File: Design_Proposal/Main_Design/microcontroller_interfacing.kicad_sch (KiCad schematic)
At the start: 9 parts, among them J12 Conn_01x02_Male, U3 CH340C, U4 M24C16-RMN6TP

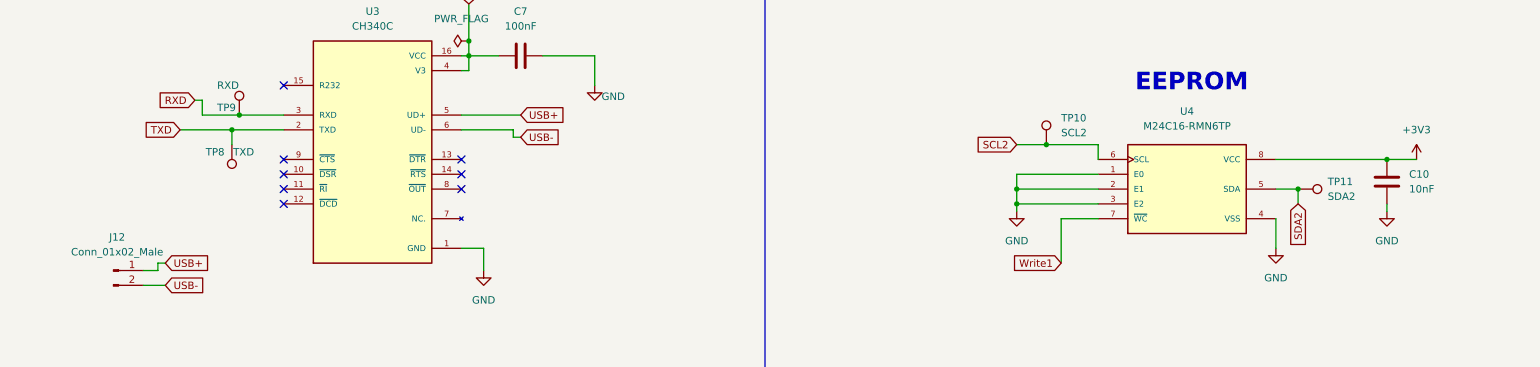
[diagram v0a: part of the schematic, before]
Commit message: update
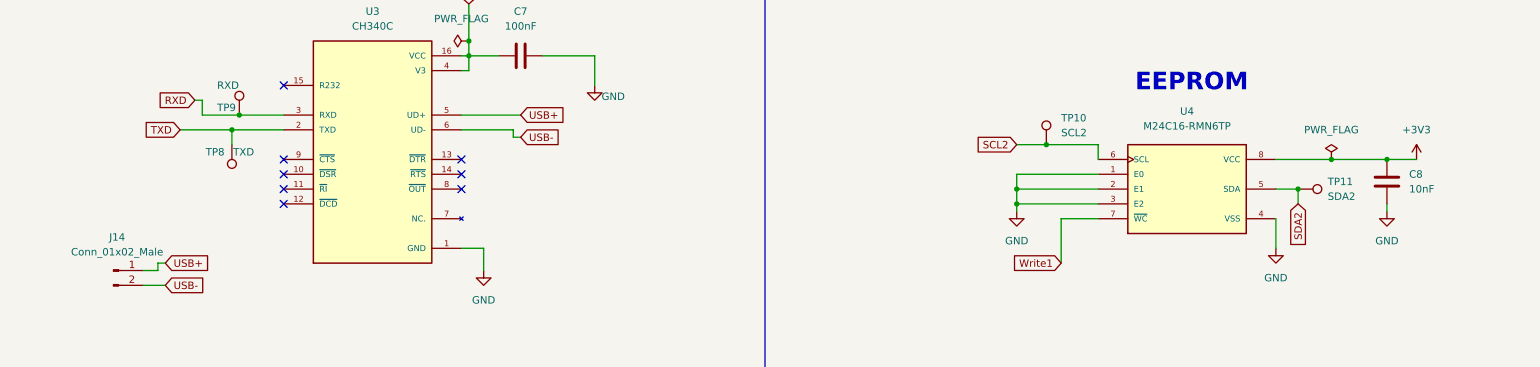
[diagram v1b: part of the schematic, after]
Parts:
- U3: footprint SOIC127P600X180-16N -> CH340:SOIC127P600X180-16N
- renumbered C10 to C8, J12 to J14
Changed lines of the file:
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@@
   (junction (at 110.49 104.14) (diameter 0) (color 0 0 0 0)
+  )
+  (junction (at 258.445 121.92) (diameter 0) (color 0 0 0 0)
   )
   (junction (at 69.85 116.84) (diameter 0) (color 0 0 0 0)
@@
     (stroke (width 0) (type default) (color 0 0 0 0))
   )
+  (wire (pts (xy 258.445 121.92) (xy 267.97 121.92))
+    (stroke (width 0) (type default) (color 0 0 0 0))
+  )
   (wire (pts (xy 78.74 114.3) (xy 71.12 114.3))
     (stroke (width 0) (type default) (color 0 0 0 0))
@@
     (stroke (width 0) (type default) (color 0 0 0 0))
   )
-  (wire (pts (xy 248.92 121.92) (xy 267.97 121.92))
+  (wire (pts (xy 248.92 121.92) (xy 258.445 121.92))
     (stroke (width 0) (type default) (color 0 0 0 0))
   )
@@
   (symbol (lib_id "Connector:Conn_01x02_Male") (at 49.53 140.97 0) (unit 1)
     (in_bom yes) (on_board yes) (fields_autoplaced)
-    (property "Reference" "J12" (id 0) (at 50.165 135.255 0))
+    (property "Reference" "J14" (id 0) (at 50.165 135.255 0))
     (property "Value" "Conn_01x02_Male" (id 1) (at 50.165 137.795 0))
     (property "Footprint" "Connector_PinHeader_2.54mm:PinHeader_1x02_P2.54mm_Vertical" (id 2) (at 49.53 140.97 0)
@@
   (symbol (lib_id "power:GND") (at 113.03 140.97 0) (unit 1)
     (in_bom yes) (on_board yes) (fields_autoplaced)
-    (property "Reference" "#PWR025" (id 0) (at 113.03 147.32 0)
+    (property "Reference" "#PWR028" (id 0) (at 113.03 147.32 0)
       (effects (font (size 1.27 1.27)) hide)
     )
@@
     (property "Reference" "U3" (id 0) (at 93.98 96.52 0))
     (property "Value" "CH340C" (id 1) (at 93.98 99.06 0))
-    (property "Footprint" "SOIC127P600X180-16N" (id 2) (at 93.98 121.92 0)
+    (property "Footprint" "CH340:SOIC127P600X180-16N" (id 2) (at 93.98 121.92 0)
       (effects (font (size 1.27 1.27)) (justify left bottom) hide)
     )
@@
   (symbol (lib_id "power:GND") (at 132.08 109.22 0) (unit 1)
     (in_bom yes) (on_board yes)
-    (property "Reference" "#PWR026" (id 0) (at 132.08 115.57 0)
+    (property "Reference" "#PWR029" (id 0) (at 132.08 115.57 0)
       (effects (font (size 1.27 1.27)) hide)
     )
@@
   (symbol (lib_id "power:GND") (at 248.92 137.16 0) (unit 1)
     (in_bom yes) (on_board yes) (fields_autoplaced)
-    (property "Reference" "#PWR030" (id 0) (at 248.92 143.51 0)
+    (property "Reference" "#PWR031" (id 0) (at 248.92 143.51 0)
       (effects (font (size 1.27 1.27)) hide)
     )
@@
   (symbol (lib_id "power:+3V3") (at 273.05 121.92 0) (unit 1)
     (in_bom yes) (on_board yes) (fields_autoplaced)
-    (property "Reference" "#PWR0106" (id 0) (at 273.05 125.73 0)
+    (property "Reference" "#PWR033" (id 0) (at 273.05 125.73 0)
       (effects (font (size 1.27 1.27)) hide)
     )
@@
     (pin "1")
   )
+  (symbol (lib_id "power:PWR_FLAG") (at 258.445 121.92 0) (unit 1)
+    (in_bom yes) (on_board yes) (fields_autoplaced)
+    (property "Reference" "#FLG06" (id 0) (at 258.445 120.015 0)
+      (effects (font (size 1.27 1.27)) hide)
+    )
+    (property "Value" "PWR_FLAG" (id 1) (at 258.445 116.84 0))
+    (property "Footprint" "" (id 2) (at 258.445 121.92 0)
+      (effects (font (size 1.27 1.27)) hide)
+    )
+    (property "Datasheet" "~" (id 3) (at 258.445 121.92 0)
+      (effects (font (size 1.27 1.27)) hide)
+    )
+    (pin "1")
+  )
   (symbol (lib_id "power:GND") (at 204.47 130.81 0) (unit 1)
     (in_bom yes) (on_board yes) (fields_autoplaced)
-    (property "Reference" "#PWR029" (id 0) (at 204.47 137.16 0)
+    (property "Reference" "#PWR030" (id 0) (at 204.47 137.16 0)
       (effects (font (size 1.27 1.27)) hide)
     )
@@
   (symbol (lib_id "Device:C") (at 267.97 125.73 0) (unit 1)
     (in_bom yes) (on_board yes) (fields_autoplaced)
-    (property "Reference" "C10" (id 0) (at 271.78 124.4599 0)
+    (property "Reference" "C8" (id 0) (at 271.78 124.4599 0)
       (effects (font (size 1.27 1.27)) (justify left))
     )
@@
   (symbol (lib_id "power:PWR_FLAG") (at 110.49 101.6 90) (unit 1)
     (in_bom yes) (on_board yes) (fields_autoplaced)
-    (property "Reference" "#FLG04" (id 0) (at 108.585 101.6 0)
+    (property "Reference" "#FLG05" (id 0) (at 108.585 101.6 0)
       (effects (font (size 1.27 1.27)) hide)
     )
@@
   (symbol (lib_id "power:GND") (at 267.97 130.81 0) (unit 1)
     (in_bom yes) (on_board yes) (fields_autoplaced)
-    (property "Reference" "#PWR031" (id 0) (at 267.97 137.16 0)
-      (effects (font (size 1.27 1.27)) hide)
-    )
+    (property "Reference" "#PWR032" (id 0) (at 267.97 137.16 0)
+      (effects (font (size 1.27 1.27)) hide)
+    )
